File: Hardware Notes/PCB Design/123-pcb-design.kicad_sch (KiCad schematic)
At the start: 2 parts, among them U1 ESP32-C3-MINI-1, U2 MCP73871

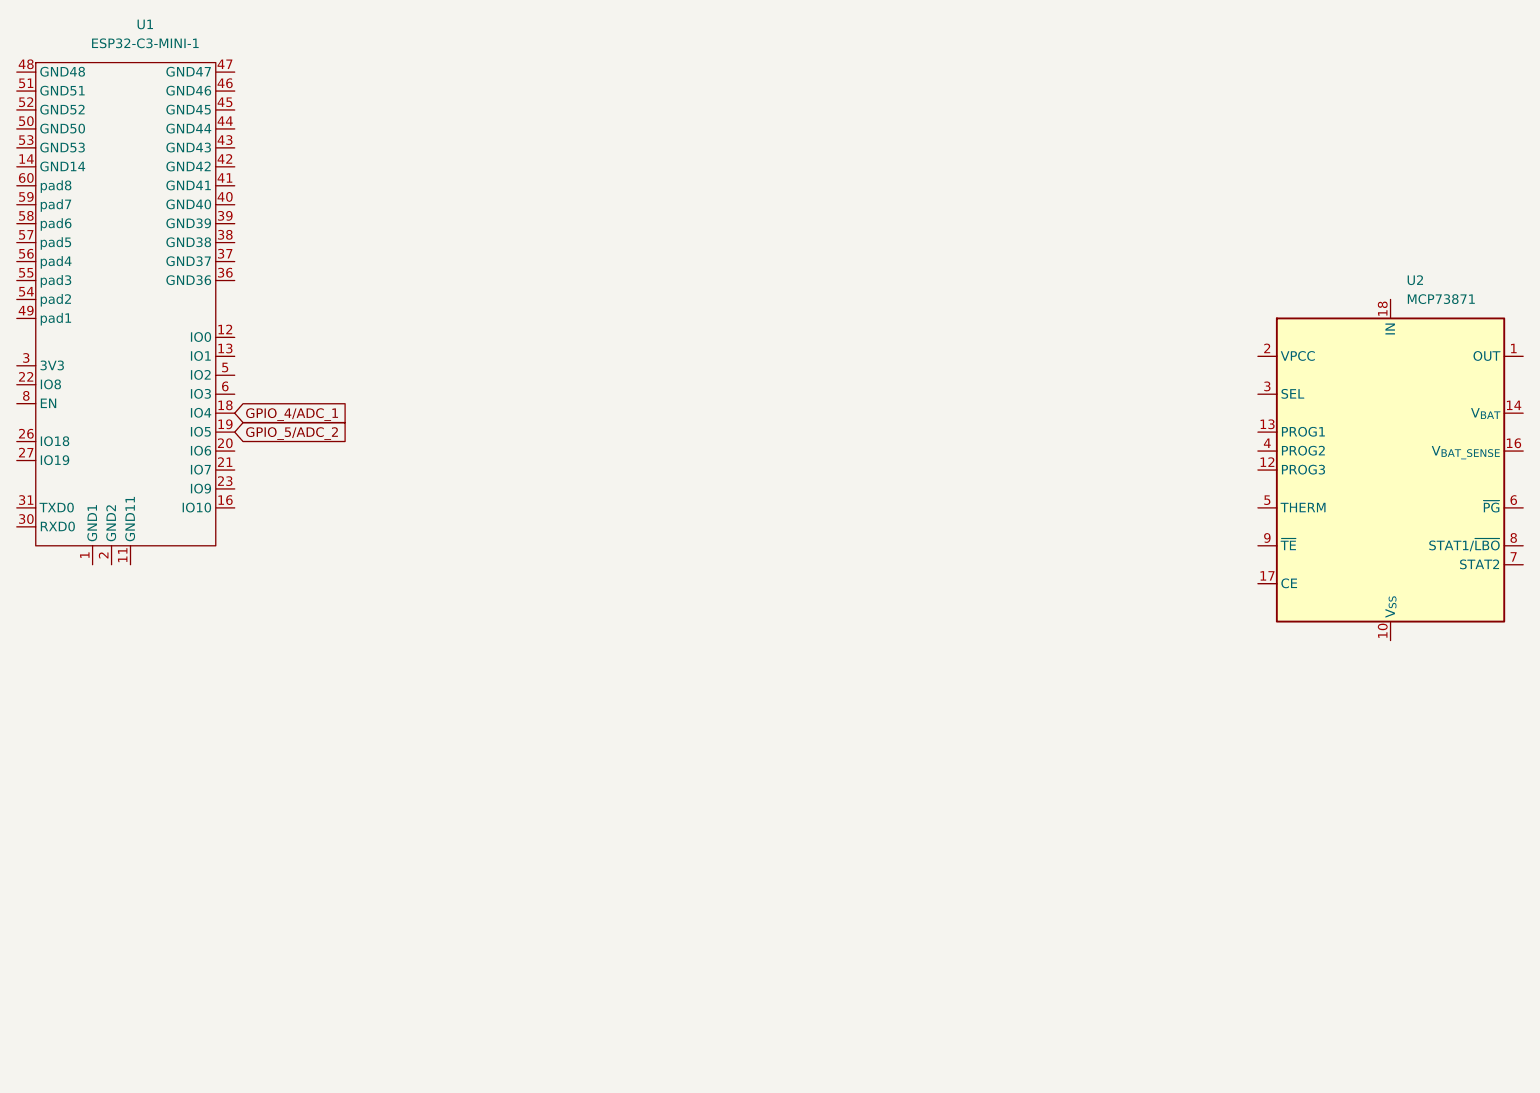
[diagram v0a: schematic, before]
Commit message: ADC file added
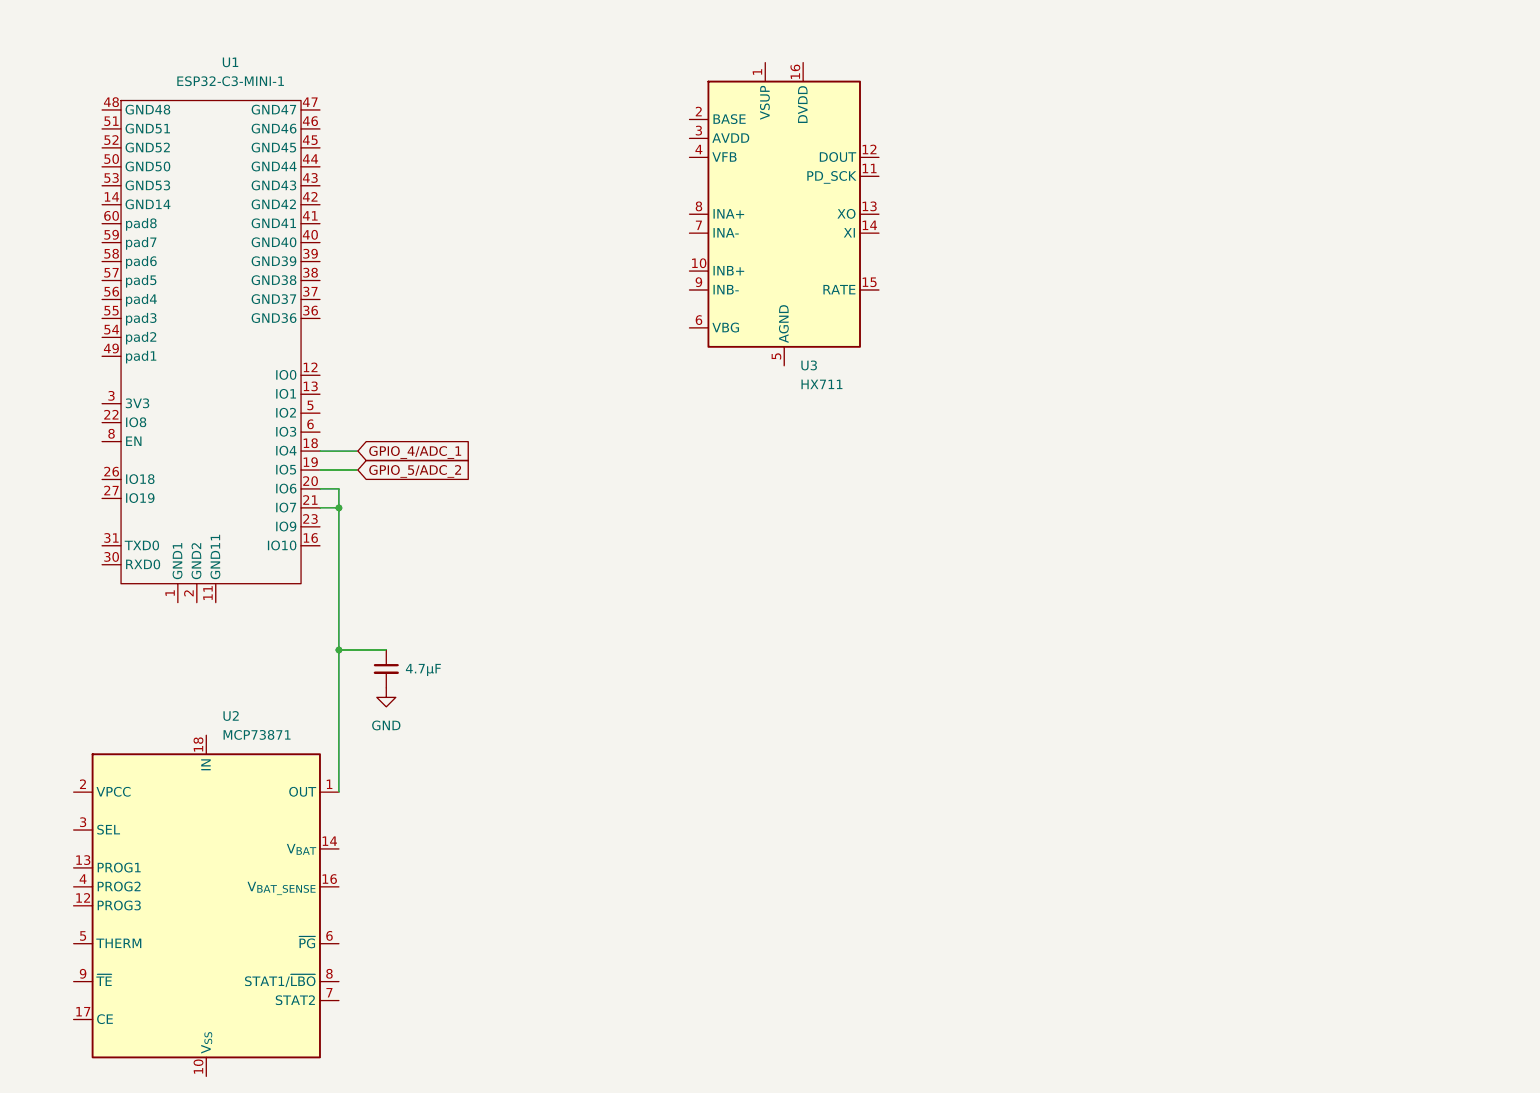
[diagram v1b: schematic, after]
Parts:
- added 4.7: 4.7μF, symbol Device:C_Small
- added U3: HX711, Package_SO:SOIC-16_3.9x9.9mm_P1.27mm, symbol Analog_ADC:HX711
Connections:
- net at U1.20 (IO6): now also U1.21 (IO7), U2.1 (OUT), U2.20 (OUT), 4.7.1
- new net GND: 4.7.2
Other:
- moved on the sheet: U1, U2
